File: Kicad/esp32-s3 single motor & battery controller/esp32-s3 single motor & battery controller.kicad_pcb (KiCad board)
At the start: 4 copper layers, 30.4 x 40.3 mm, 132 parts, among them J1 JST SH SM04B, J2 7 pin FPC 0.3mm, J3 Conn_01x03, J4 Conn_01x03, J5 Batt Balance connector, Q1 NMOS,12v, Q2 NMOS, 12v, Q3 NMOS,12v,PPak, Q4 NMOS, 12v, Q5 NMOS, 12v, Q7 NMOS,12v,PPak, SW1 SW_Push, SW2 SW_Push, U2 AP63203WU, U3 BQ76905RGRR, U4 BQ24780SRUYR, U5 ESP32-S3, U6 74HC595, Y1 40mhz, 10ppm

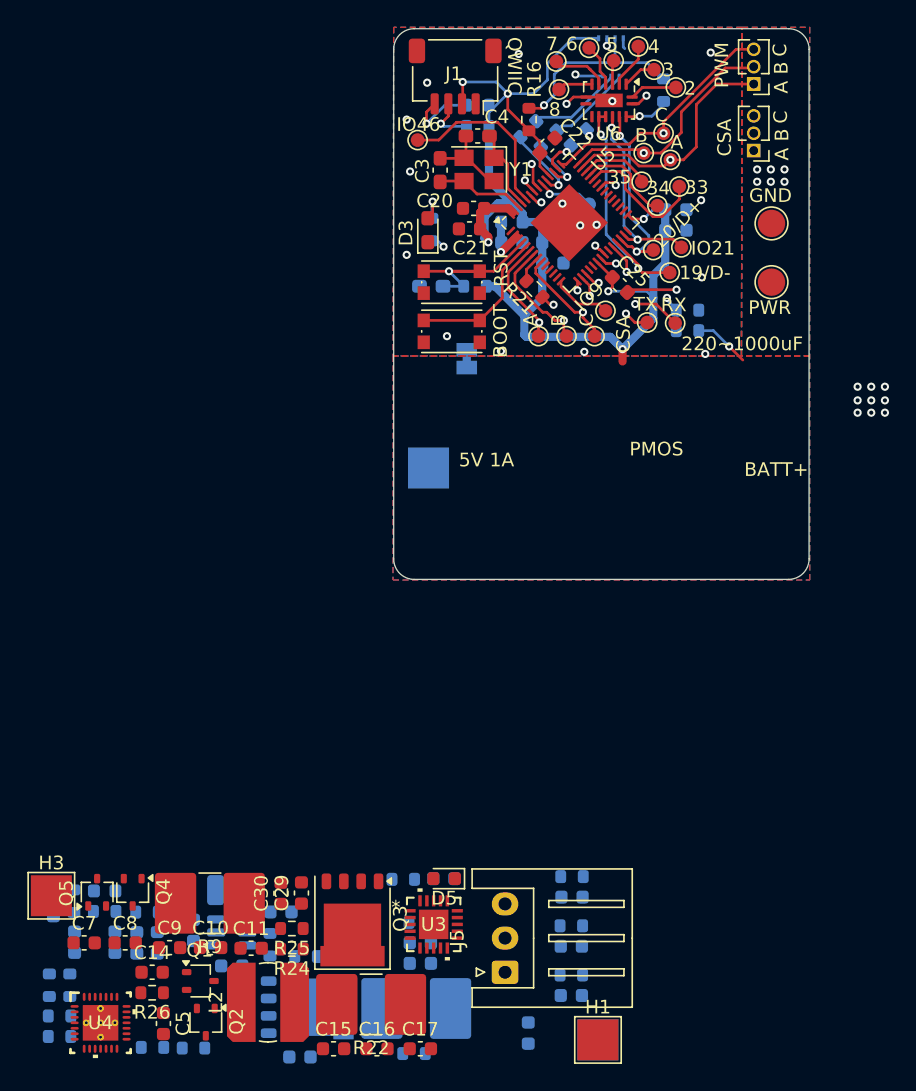
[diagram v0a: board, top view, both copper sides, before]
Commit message: Started wiring
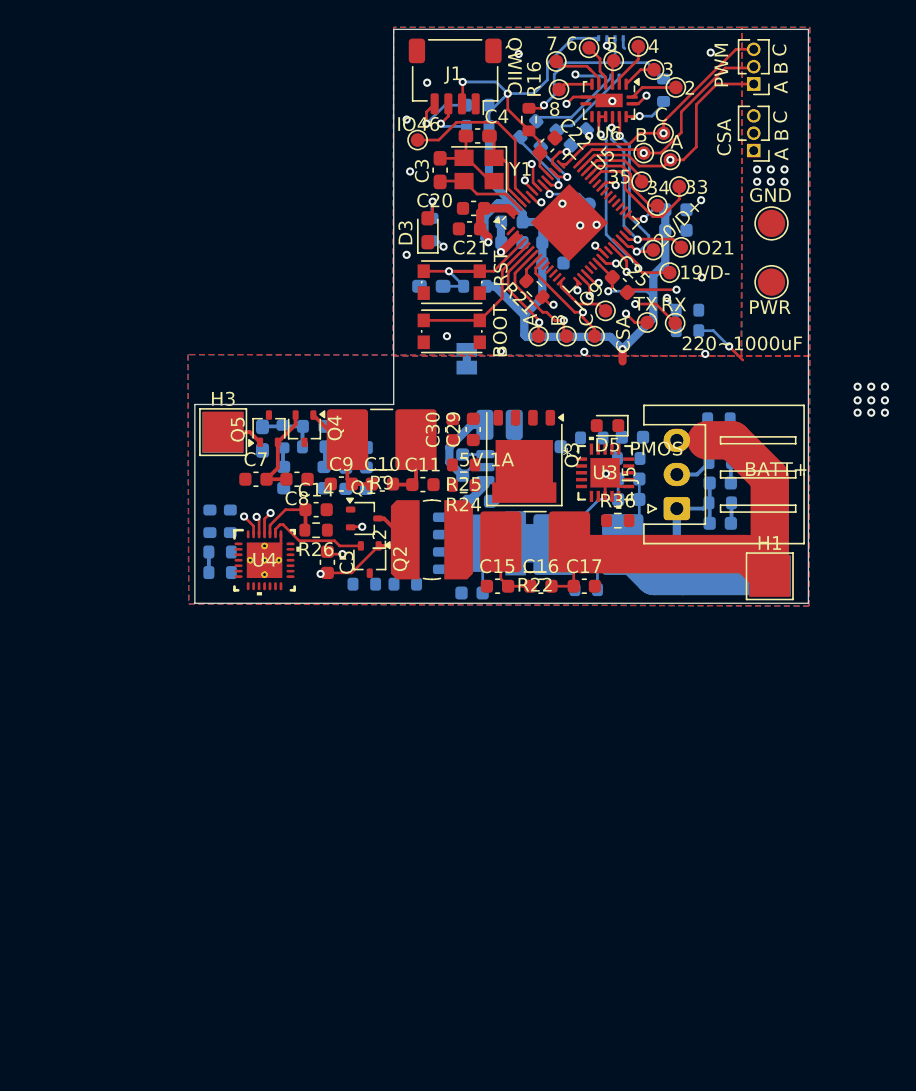
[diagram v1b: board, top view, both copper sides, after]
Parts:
- R36: moved to F.Cu
- moved C36 42.1 mm to (150.4, 125.4)
- moved R32 39.3 mm to (133.3, 122.9)
- moved L3 39.3 mm to (130.4, 118.9)
- moved U2 39.3 mm to (130.5, 122.0)
- moved C27 39.3 mm to (134.1, 120.5)
- moved C40 39.3 mm to (127.7, 121.9)
- moved R36 39.2 mm to (139.1, 126.0), turned to 0 degrees
- moved R23 38.6 mm to (123.5, 130.6), turned to 180 degrees
- moved C28 38.5 mm to (128.9, 124.5)
- moved C31 37.3 mm to (117.5, 122.8)
- moved C6 37.3 mm to (114.6, 122.8)
- moved D2 37.3 mm to (116.8, 119.0)
- moved R11 37.3 mm to (114.5, 119.8)
- moved R28 37.3 mm to (116.8, 120.5)
- moved C12 37.3 mm to (119.2, 122.8)
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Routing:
- net /PSU/BATT+: track 0.00 -> 41.9 mm
- net /PSU/BATT-: track 0.00 -> 31.7 mm
- net Net-(Q1-S): track 0.00 -> 18.8 mm, vias 0 -> 2
- net Net-(Q7-S): track 0.00 -> 18.5 mm
- net Net-(Q1-G): track 0.00 -> 11.0 mm, vias 0 -> 2
- net Net-(U4-BTST): track 0.00 -> 9.42 mm, vias 0 -> 2
- net /MOTORPWR: track 4.12 -> 13.5 mm
- net Net-(Q4-D): track 0.00 -> 8.07 mm
- net Net-(U2-SW): track 0.00 -> 7.69 mm
- net /PSU/IN: track 0.00 -> 7.50 mm
- net Net-(Q2-G): track 0.00 -> 7.40 mm
- net GNDPWR: track 1.27 -> 8.32 mm, vias 15 -> 16
- net Net-(Q4-G): track 0.00 -> 7.03 mm
- net Net-(D2-K): track 0.00 -> 5.27 mm
- net /PSU/REGN: track 0.00 -> 5.26 mm
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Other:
- board size 30.4 x 40.3 mm -> 44.9 x 42 mm
